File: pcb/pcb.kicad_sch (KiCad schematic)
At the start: 8 parts, among them U1 1117-3.3

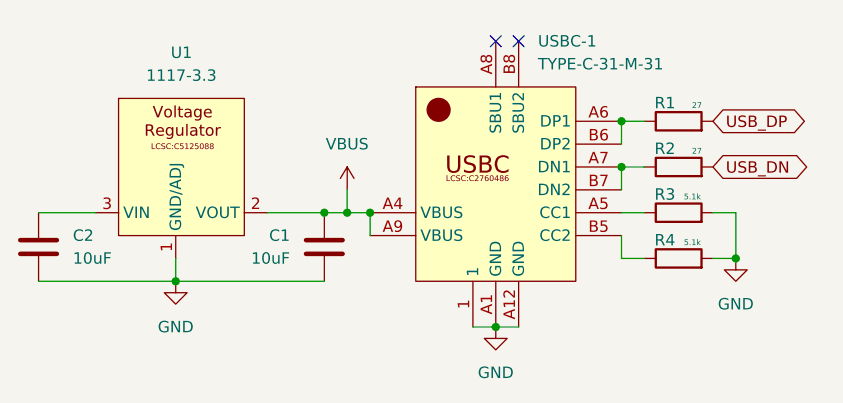
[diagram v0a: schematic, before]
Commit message: fixxed usbc stuff
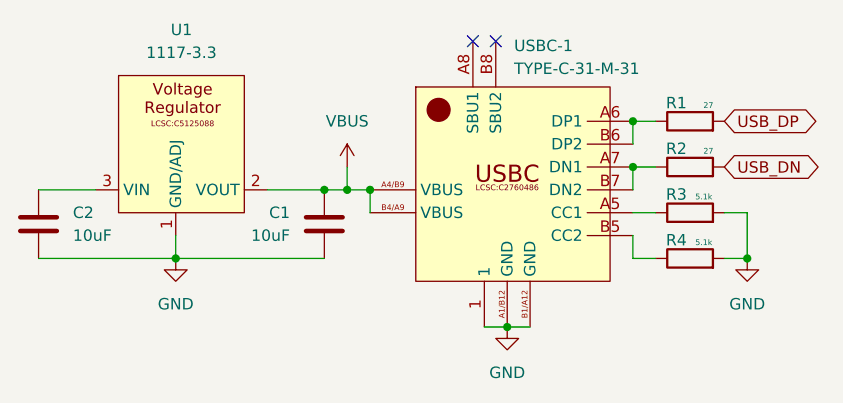
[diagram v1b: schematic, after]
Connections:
- net GND: now also USBC-1.A1/B12 (GND), USBC-1.B1/A12 (GND); no longer USBC-1.A1 (GND), USBC-1.A12 (GND)
- net VBUS: now also USBC-1.A4/B9 (VBUS), USBC-1.B4/A9 (VBUS); no longer USBC-1.A4 (VBUS), USBC-1.A9 (VBUS)
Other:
- moved on the sheet: C1, C2, R1, R2, R3, R4, U1, USBC-1
